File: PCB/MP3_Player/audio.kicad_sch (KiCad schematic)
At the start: 23 parts, among them J4 SJ3-35044A, J9 SJ3-35044A, U6 PCM5102AQPWRQ1

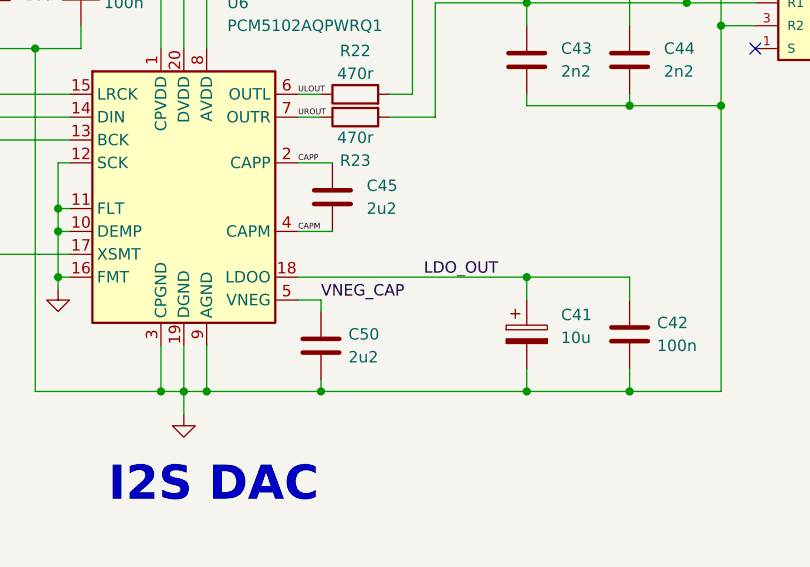
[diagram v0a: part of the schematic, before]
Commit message: Final PCB Routing
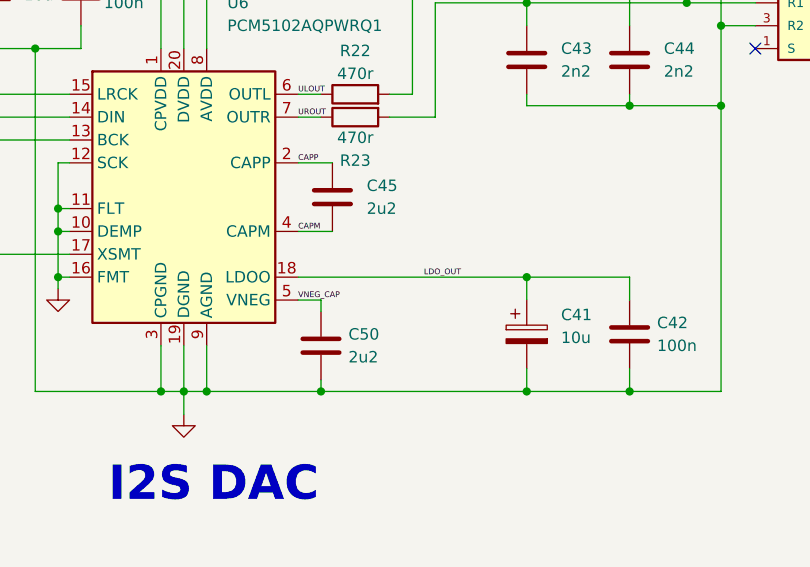
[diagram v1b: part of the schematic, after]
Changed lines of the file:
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@@
-	(wire
-		(pts
-			(xy 168.91 102.87) (xy 168.91 104.14)
-		)
-		(stroke
-			(width 0)
-			(type default)
-		)
-	)
 	(wire
 		(pts
@@
 	(wire
 		(pts
+			(xy 168.91 104.14) (xy 168.91 102.87)
+		)
+		(stroke
+			(width 0)
+			(type default)
+		)
+	)
+	(wire
+		(pts
 			(xy 203.2 80.01) (xy 203.2 81.28)
 		)
@@
 	(wire
 		(pts
+			(xy 168.91 102.87) (xy 166.37 102.87)
+		)
+		(stroke
+			(width 0)
+			(type default)
+		)
+	)
+	(wire
+		(pts
 			(xy 166.37 87.63) (xy 170.18 87.63)
 		)
@@
 		(pts
 			(xy 92.71 105.41) (xy 92.71 153.67)
-		)
-		(stroke
-			(width 0)
-			(type default)
-		)
-	)
-	(wire
-		(pts
-			(xy 166.37 102.87) (xy 168.91 102.87)
 		)
 		(stroke
@@
 		(effects
 			(font
-				(size 1.27 1.27)
+				(size 0.635 0.635)
 			)
 			(justify left bottom)
@@
 	)
 	(label "VNEG_CAP"
-		(at 168.91 102.87 0)
+		(at 166.37 102.87 0)
 		(effects
 			(font
-				(size 1.27 1.27)
+				(size 0.635 0.635)
 			)
 			(justify left bottom)
